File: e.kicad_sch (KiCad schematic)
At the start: 10 parts, among them SW1 usr, SW2 rst, U1 Display_ST7789, U2 MAX98357A

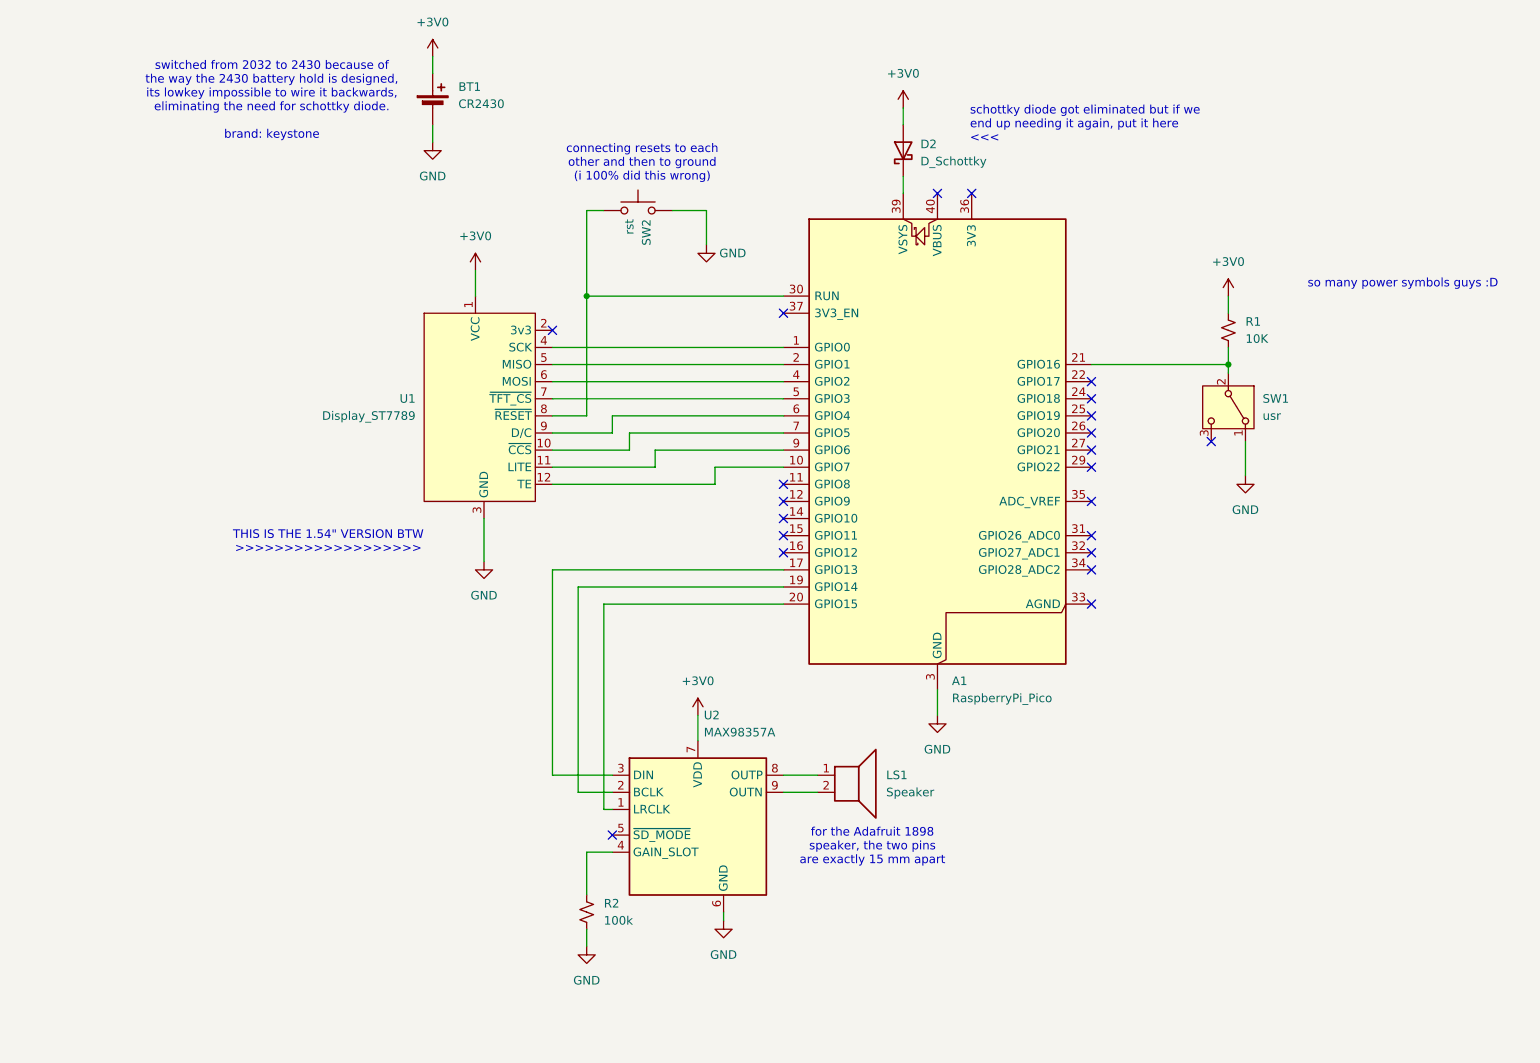
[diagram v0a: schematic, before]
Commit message: wowwwww
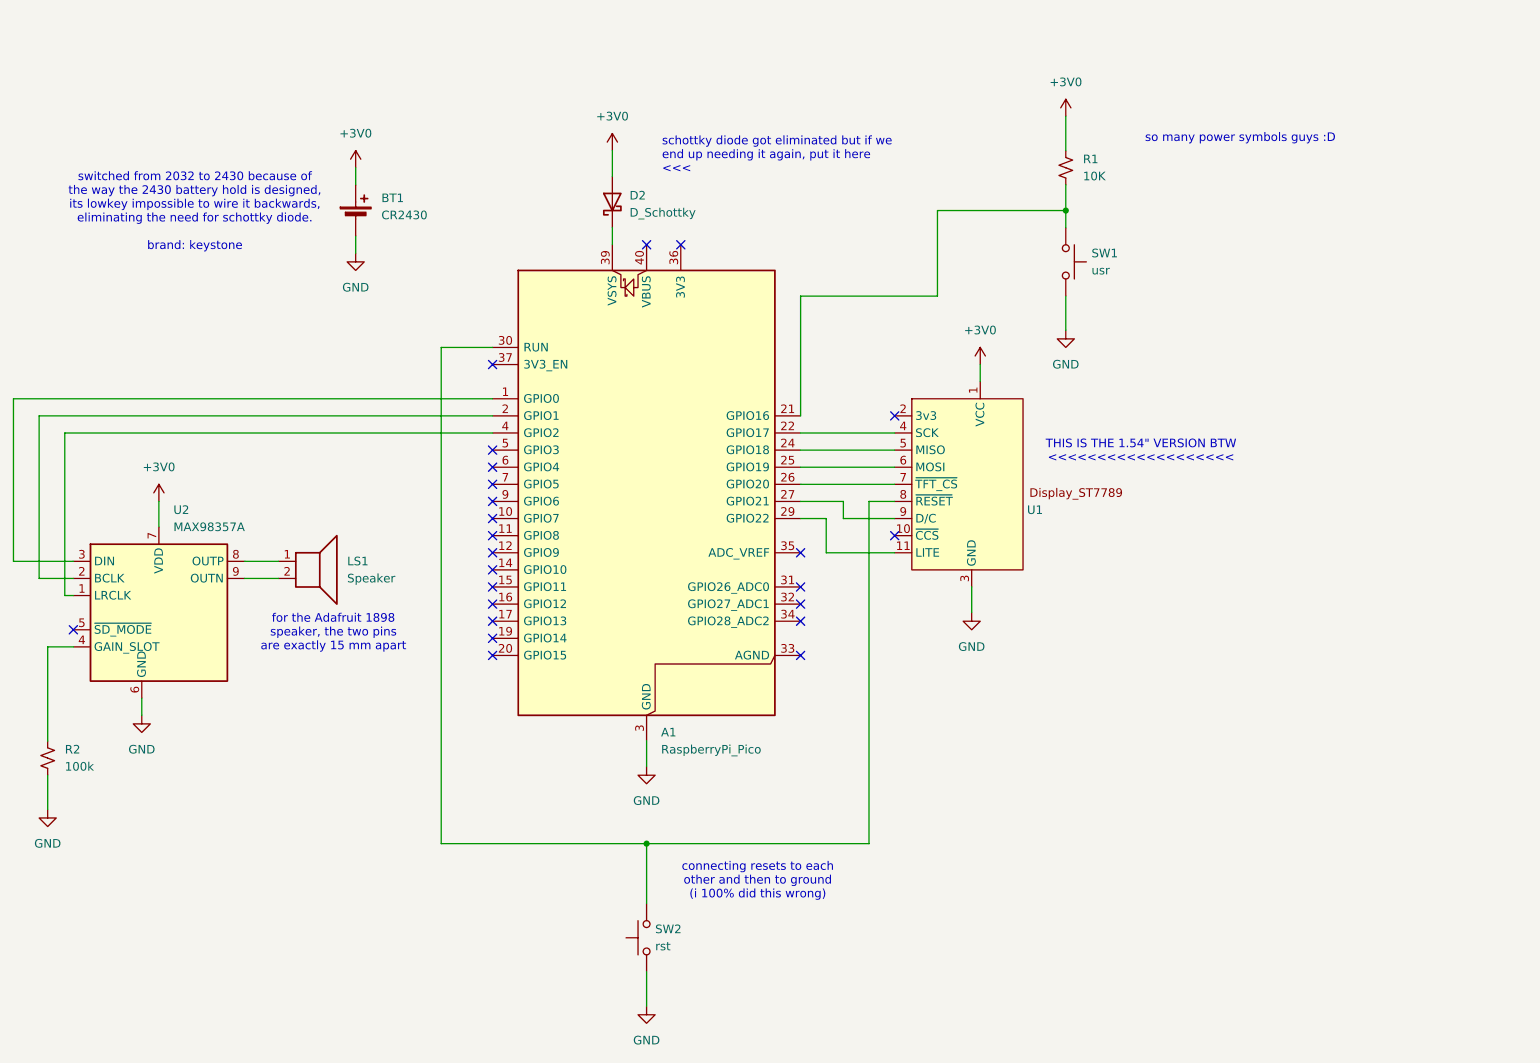
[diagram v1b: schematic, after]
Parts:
- removed SW1: usr, Button_Switch_THT:SW_Slide_SPDT_Straight_CK_OS102011MS2Q, symbol Switch:SW_SPDT
- removed U1: Display_ST7789, custom-fp:display-lol, symbol cool-stuff:small-display
- added SW1: usr, Button_Switch_SMD:SW_SPST_B3S-1000, symbol Switch:SW_Push
- added U1: (no value), display-lol:display-lol, symbol display_idk_lol:small-display
- LS1: footprint custom-fp:stupid-dumb-speaker -> stupid-dumb-speaker:stupid-dumb-speaker
- U2: footprint custom-fp:MAX98357A -> Package_DFN_QFN:TQFN-16-1EP_3x3mm_P0.5mm_EP1.23x1.23mm
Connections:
- net +3V0: now also U2.8 (OUTP), U1.1 (VCC)
- net GND: now also SW2.1, U2.11 (GND), U2.15 (GND), SW1.2, U1.3 (GND); no longer SW2.2
- net at A1.20 (GPIO15): no longer U2.1 (LRCLK)
- net at A1.19 (GPIO14): no longer U2.2 (BCLK)
- net at U2.3 (DIN): now also A1.1 (GPIO0); no longer A1.17 (GPIO13)
- net at A1.2 (GPIO1): now also U2.2 (BCLK)
- net at A1.21 (GPIO16), R1.2: now also SW1.1
- net at A1.22 (GPIO17): now also U1.4 (SCK)
- net at A1.24 (GPIO18): now also U1.5 (MISO)
- net at A1.25 (GPIO19): now also U1.6 (MOSI)
- net at A1.26 (GPIO20): now also U1.7 (~{TFT_CS})
- net at A1.27 (GPIO21): now also U1.9 (D/C)
- net at A1.29 (GPIO22): now also U1.11 (LITE)
- net at A1.30 (RUN): now also SW2.2, U1.8 (~{RESET}); no longer SW2.1
- net at A1.4 (GPIO2): now also U2.1 (LRCLK)
- no-connect marks 22 -> 24
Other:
- note added: "THIS IS THE 1.54" VERSION BTW <<<<<<<<<<<<<<<<<<<"
- note removed: "THIS IS THE 1.54" VERSION BTW >>>>>>>>>>>>>>>>>>>"
- moved on the sheet: A1, BT1, D2, LS1, R1, R2
